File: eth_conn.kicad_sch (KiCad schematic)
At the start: 23 parts, among them J1 RJ45

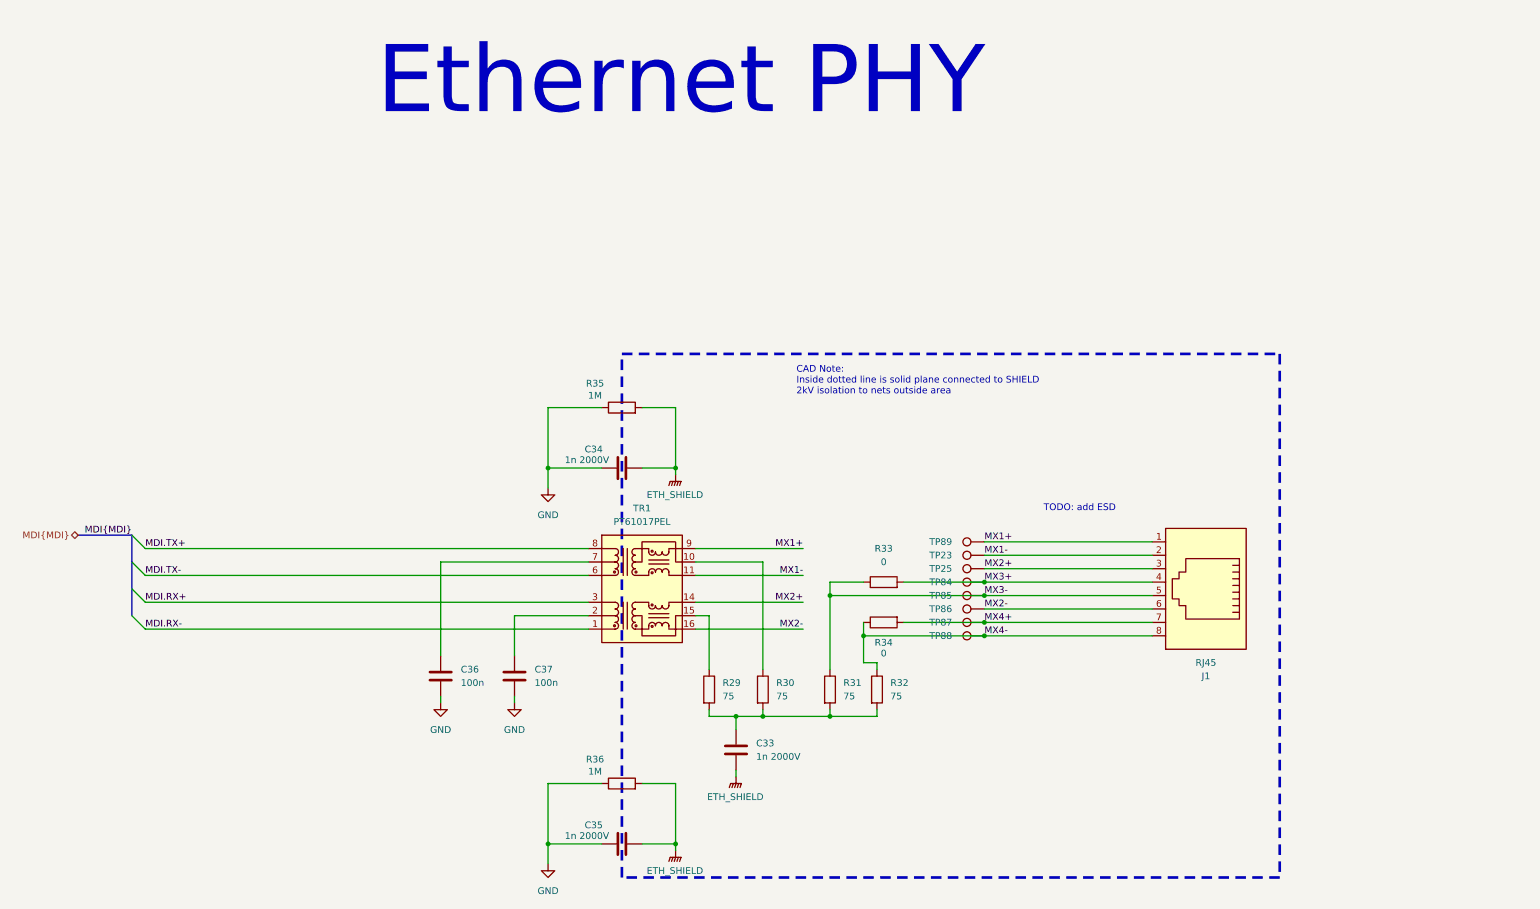
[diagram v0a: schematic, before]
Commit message: did stuff
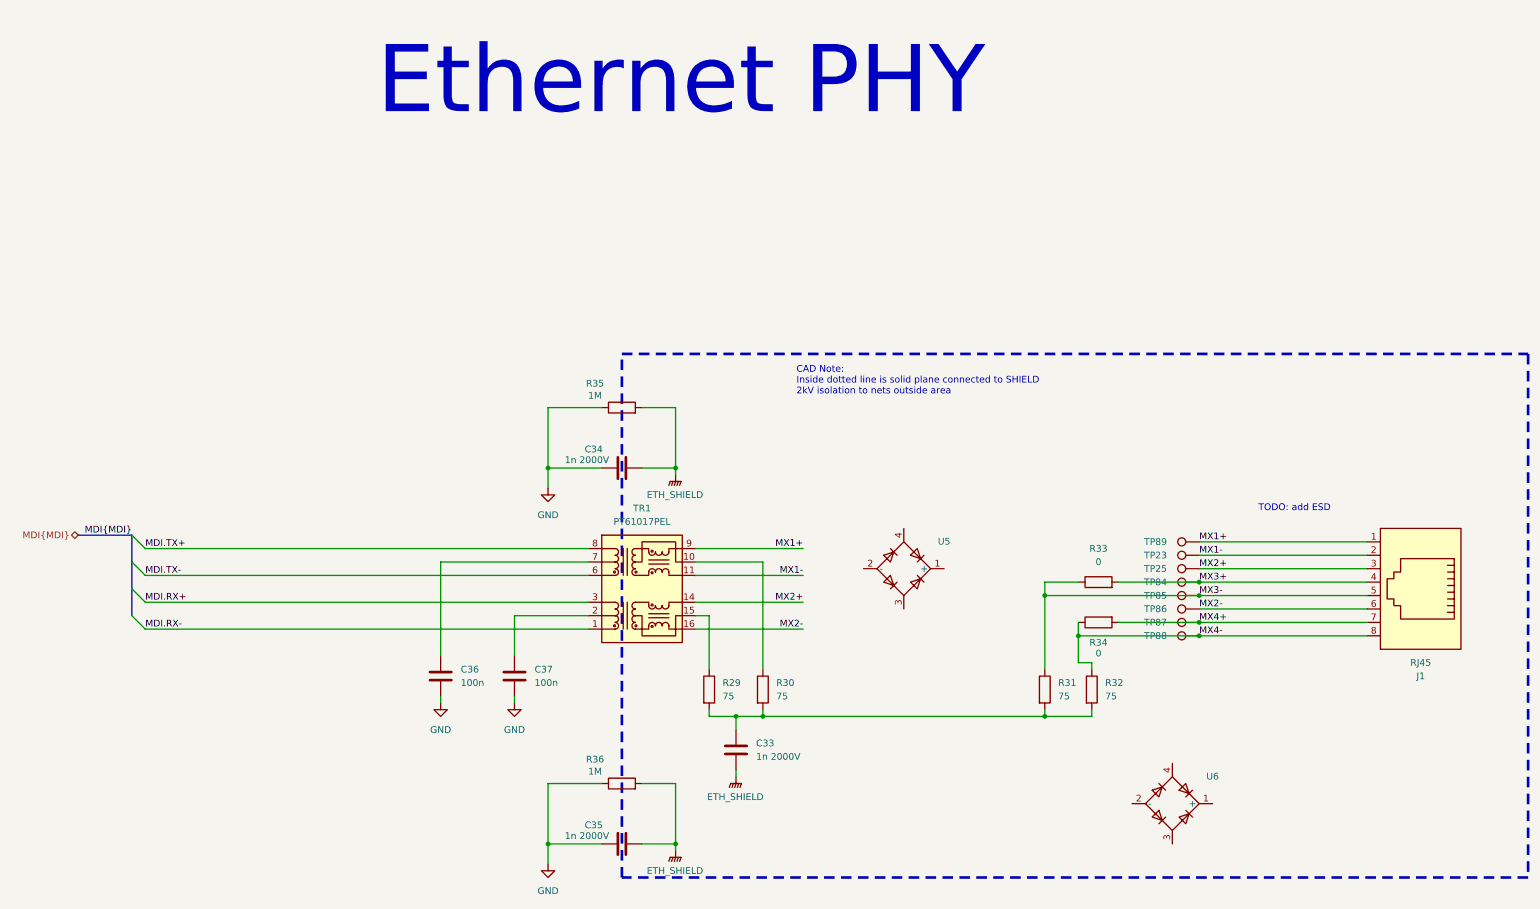
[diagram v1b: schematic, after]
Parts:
- added U5, U6: ~, CDHD01:CDHD01, symbol CDHD01:CDHD01
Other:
- moved on the sheet: J1, R31, R32, R33, R34, TP23, TP25, TP84, TP85, TP86, TP87, TP88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
